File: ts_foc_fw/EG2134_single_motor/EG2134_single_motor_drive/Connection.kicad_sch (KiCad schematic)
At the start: 3 parts, among them CN1 XT30PW-M, CN2 WAFER-GH1.25-10PWB, U5 MR30PW-M30.G.Y

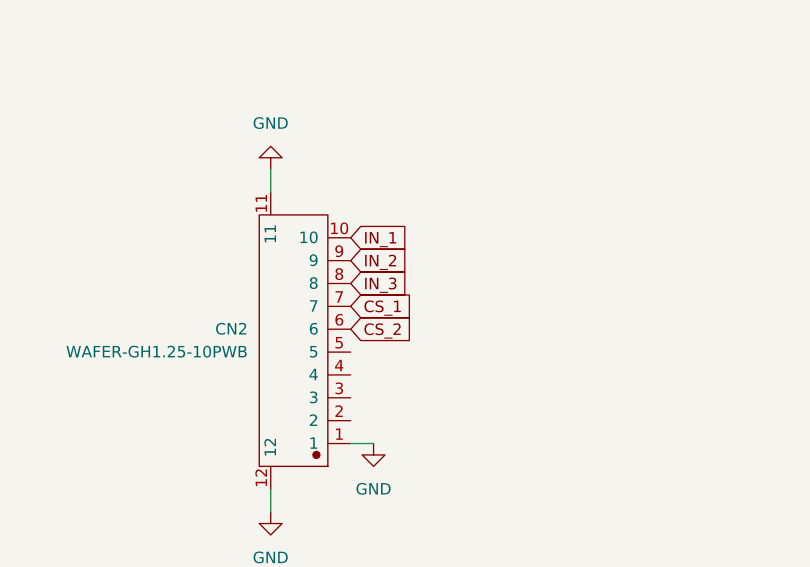
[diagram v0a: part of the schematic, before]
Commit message: tongbu
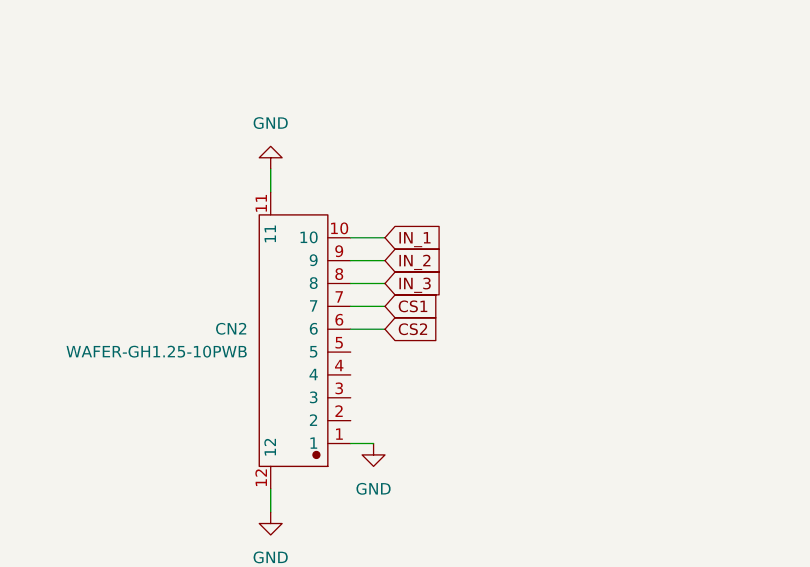
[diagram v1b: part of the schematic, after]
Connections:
- net CS_1 renamed CS1
- net CS_2 renamed CS2
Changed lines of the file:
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@@
+	(wire
+		(pts
+			(xy 90.17 100.33) (xy 86.36 100.33)
+		)
+		(stroke
+			(width 0)
+			(type default)
+		)
+	)
+	(wire
+		(pts
+			(xy 90.17 102.87) (xy 86.36 102.87)
+		)
+		(stroke
+			(width 0)
+			(type default)
+		)
+	)
 	(wire
 		(pts
@@
 	(wire
 		(pts
+			(xy 90.17 107.95) (xy 86.36 107.95)
+		)
+		(stroke
+			(width 0)
+			(type default)
+		)
+	)
+	(wire
+		(pts
+			(xy 90.17 110.49) (xy 86.36 110.49)
+		)
+		(stroke
+			(width 0)
+			(type default)
+		)
+	)
+	(wire
+		(pts
 			(xy 138.43 45.72) (xy 138.43 48.26)
 		)
@@
 		(pts
 			(xy 77.47 130.81) (xy 77.47 128.27)
+		)
+		(stroke
+			(width 0)
+			(type default)
+		)
+	)
+	(wire
+		(pts
+			(xy 90.17 105.41) (xy 86.36 105.41)
 		)
 		(stroke
@@
 		)
 	)
-	(global_label "CS_1"
-		(shape input)
-		(at 86.36 107.95 0)
-		(fields_autoplaced yes)
-		(effects
-			(font
-				(size 1.27 1.27)
-			)
-			(justify left)
-		)
-		(property "Intersheetrefs" "${INTERSHEET_REFS}"
-			(at 94.0018 107.95 0)
+	(global_label "CS1"
+		(shape input)
+		(at 90.17 107.95 0)
+		(fields_autoplaced yes)
+		(effects
+			(font
+				(size 1.27 1.27)
+			)
+			(justify left)
+		)
+		(property "Intersheetrefs" "${INTERSHEET_REFS}"
+			(at 96.8442 107.95 0)
 			(effects
 				(font
@@
 	(global_label "IN_2"
 		(shape input)
-		(at 86.36 102.87 0)
-		(fields_autoplaced yes)
-		(effects
-			(font
-				(size 1.27 1.27)
-			)
-			(justify left)
-		)
-		(property "Intersheetrefs" "${INTERSHEET_REFS}"
-			(at 93.4576 102.87 0)
-			(effects
-				(font
-					(size 1.27 1.27)
-				)
-				(justify left)
-				(hide yes)
-			)
-		)
-	)
-	(global_label "CS_2"
-		(shape input)
-		(at 86.36 110.49 0)
-		(fields_autoplaced yes)
-		(effects
-			(font
-				(size 1.27 1.27)
-			)
-			(justify left)
-		)
-		(property "Intersheetrefs" "${INTERSHEET_REFS}"
-			(at 94.0018 110.49 0)
+		(at 90.17 102.87 0)
+		(fields_autoplaced yes)
+		(effects
+			(font
+				(size 1.27 1.27)
+			)
+			(justify left)
+		)
+		(property "Intersheetrefs" "${INTERSHEET_REFS}"
+			(at 97.2676 102.87 0)
+			(effects
+				(font
+					(size 1.27 1.27)
+				)
+				(justify left)
+				(hide yes)
+			)
+		)
+	)
+	(global_label "CS2"
+		(shape input)
+		(at 90.17 110.49 0)
+		(fields_autoplaced yes)
+		(effects
+			(font
+				(size 1.27 1.27)
+			)
+			(justify left)
+		)
+		(property "Intersheetrefs" "${INTERSHEET_REFS}"
+			(at 96.8442 110.49 0)
 			(effects
 				(font
@@
 	(global_label "IN_3"
 		(shape input)
-		(at 86.36 105.41 0)
-		(fields_autoplaced yes)
-		(effects
-			(font
-				(size 1.27 1.27)
-			)
-			(justify left)
-		)
-		(property "Intersheetrefs" "${INTERSHEET_REFS}"
-			(at 93.4576 105.41 0)
+		(at 90.17 105.41 0)
+		(fields_autoplaced yes)
+		(effects
+			(font
+				(size 1.27 1.27)
+			)
+			(justify left)
+		)
+		(property "Intersheetrefs" "${INTERSHEET_REFS}"
+			(at 97.2676 105.41 0)
 			(effects
 				(font
@@
 	(global_label "IN_1"
 		(shape input)
-		(at 86.36 100.33 0)
-		(fields_autoplaced yes)
-		(effects
-			(font
-				(size 1.27 1.27)
-			)
-			(justify left)
-		)
-		(property "Intersheetrefs" "${INTERSHEET_REFS}"
-			(at 93.4576 100.33 0)
-			(effects
-				(font
+		(at 90.17 100.33 0)
+		(fields_autoplaced yes)
+		(effects
+			(font
+				(size 1.27 1.27)
+			)
+			(justify left)
+		)
+		(property "Intersheetrefs" "${INTERSHEET_REFS}"
+			(at 97.2676 100.33 0)
+			(effects
+				(font
